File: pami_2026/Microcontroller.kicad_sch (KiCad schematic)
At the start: 11 parts, among them U1 ESP32-WROOM-E

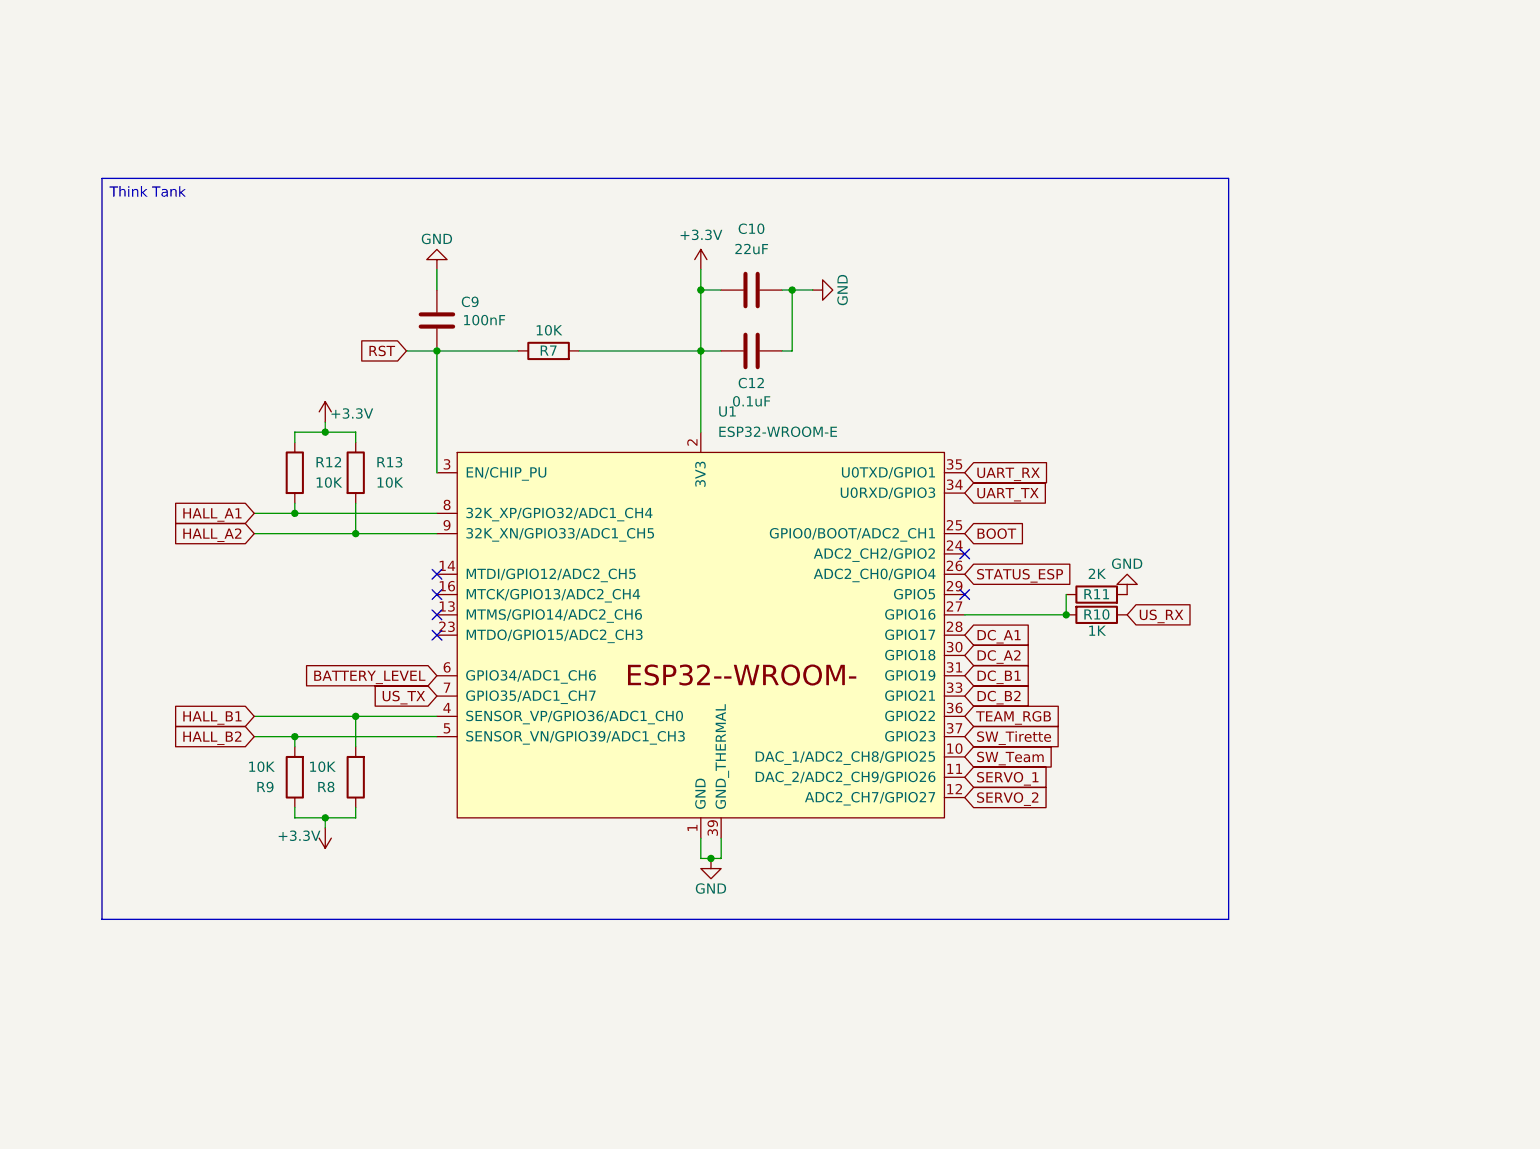
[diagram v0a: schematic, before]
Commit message: Cleanup
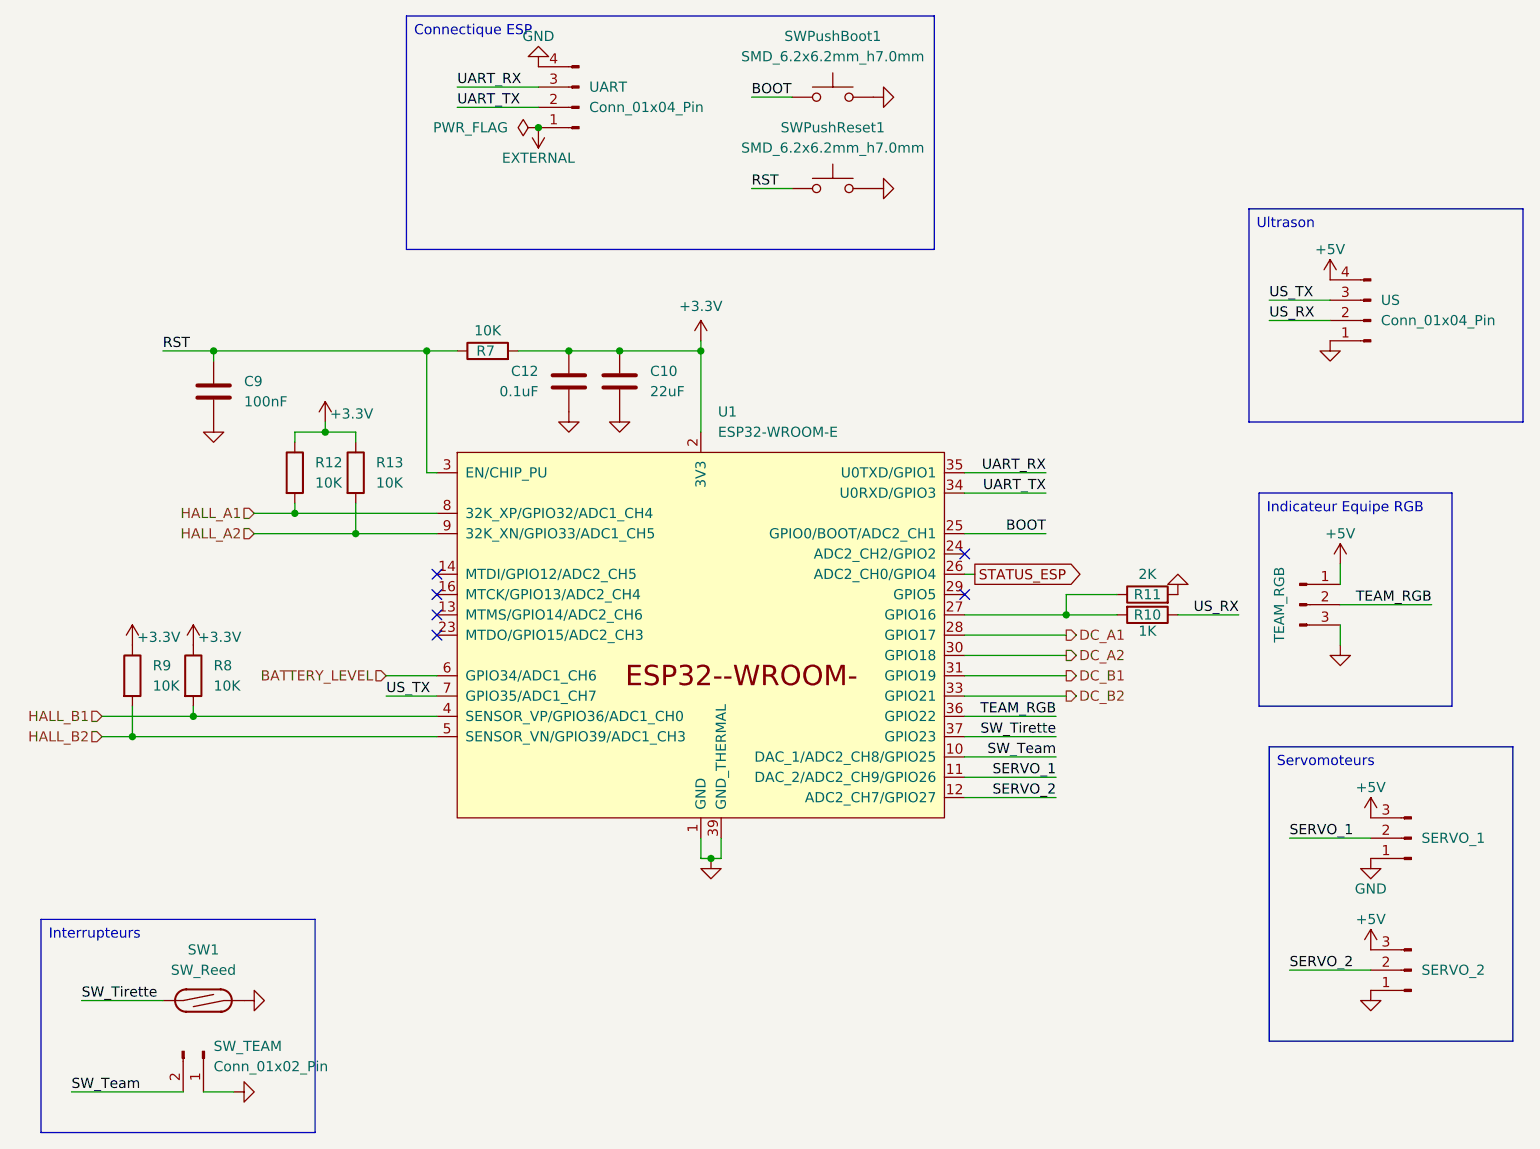
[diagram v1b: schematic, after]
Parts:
- added SERVO_1, SERVO_2, TEAM_RGB: Conn_01x03_Pin, Connector_PinHeader_2.54mm:PinHeader_1x03_P2.54mm_Vertical, symbol Connector:Conn_01x03_Pin
- added SW1: SW_Reed, Connector_PinHeader_2.54mm:PinHeader_1x02_P2.54mm_Vertical, symbol Switch:SW_Reed
- added SWPushBoot1, SWPushReset1: SMD_6.2x6.2mm_h7.0mm, PCM_SparkFun-Switch:Push_SMD_6.2x6.2mm, symbol PCM_SparkFun-Switch:SPST_Push_SMD_6.2x6.2mm_h7.0mm
- added SW_TEAM: Conn_01x02_Pin, Connector_PinHeader_2.54mm:PinHeader_1x02_P2.54mm_Vertical, symbol Connector:Conn_01x02_Pin
- added UART, US: Conn_01x04_Pin, Connector_PinHeader_2.54mm:PinHeader_1x04_P2.54mm_Vertical, symbol Connector:Conn_01x04_Pin
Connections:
- net BOOT: now also SWPushBoot1.1
- net GND: now also SERVO_1.1 (Pin_1), SERVO_2.1 (Pin_1), SW1.2, SWPushBoot1.2, SWPushReset1.2, SW_TEAM.1 (Pin_1), TEAM_RGB.3 (Pin_3), UART.4 (Pin_4), US.1 (Pin_1)
- net RST: now also SWPushReset1.1
- net SERVO_1: now also SERVO_1.2 (Pin_2)
- net SERVO_2: now also SERVO_2.2 (Pin_2)
- net SW_Team: now also SW_TEAM.2 (Pin_2)
- net SW_Tirette: now also SW1.1
- net TEAM_RGB: now also TEAM_RGB.2 (Pin_2)
- net UART_RX: now also UART.3 (Pin_3)
- net UART_TX: now also UART.2 (Pin_2)
- net US_RX: now also US.2 (Pin_2)
- net US_TX: now also US.3 (Pin_3)
- new net +5V: SERVO_1.3 (Pin_3), SERVO_2.3 (Pin_3), TEAM_RGB.1 (Pin_1), US.4 (Pin_4)
- new net EXTERNAL: UART.1 (Pin_1)
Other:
- moved on the sheet: C10, C12, C9, R10, R11, R7, R8, R9
